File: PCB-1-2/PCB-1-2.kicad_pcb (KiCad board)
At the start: 2 copper layers, 51.3 x 8.4 mm, 37 parts, among them J1 Bus_PCI_Express_x8, U1 LTC1298IS8_PBF, U2 LTC1451IS8-PBF, U3 HI-3110PSIF, U4 FT231XS-R, U5 STM32F103RBT6, U6 STWD100YNXWY3F, U7 ADP7104ACPZ-5V, U8 ADP7104ACPZ-3.3V, Y1 8MHz Crystal

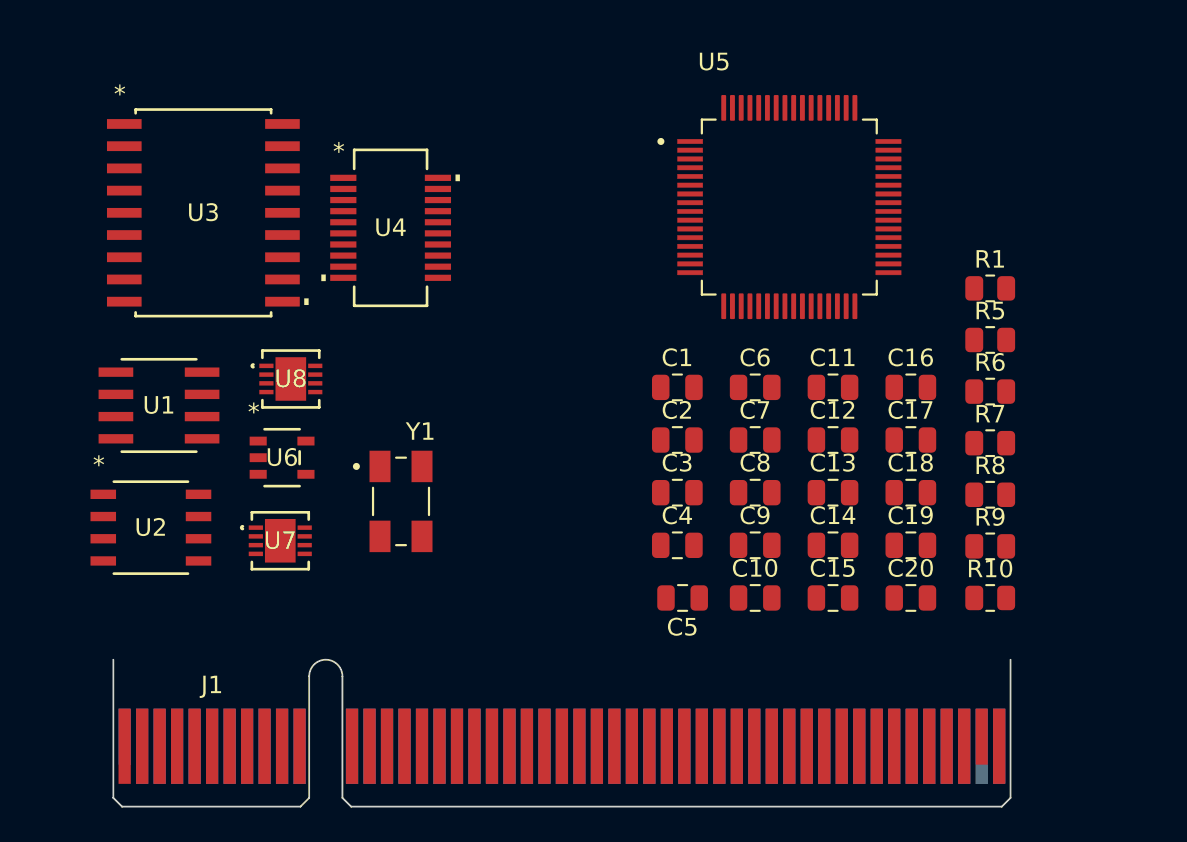
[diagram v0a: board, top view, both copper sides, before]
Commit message: Updated a few things
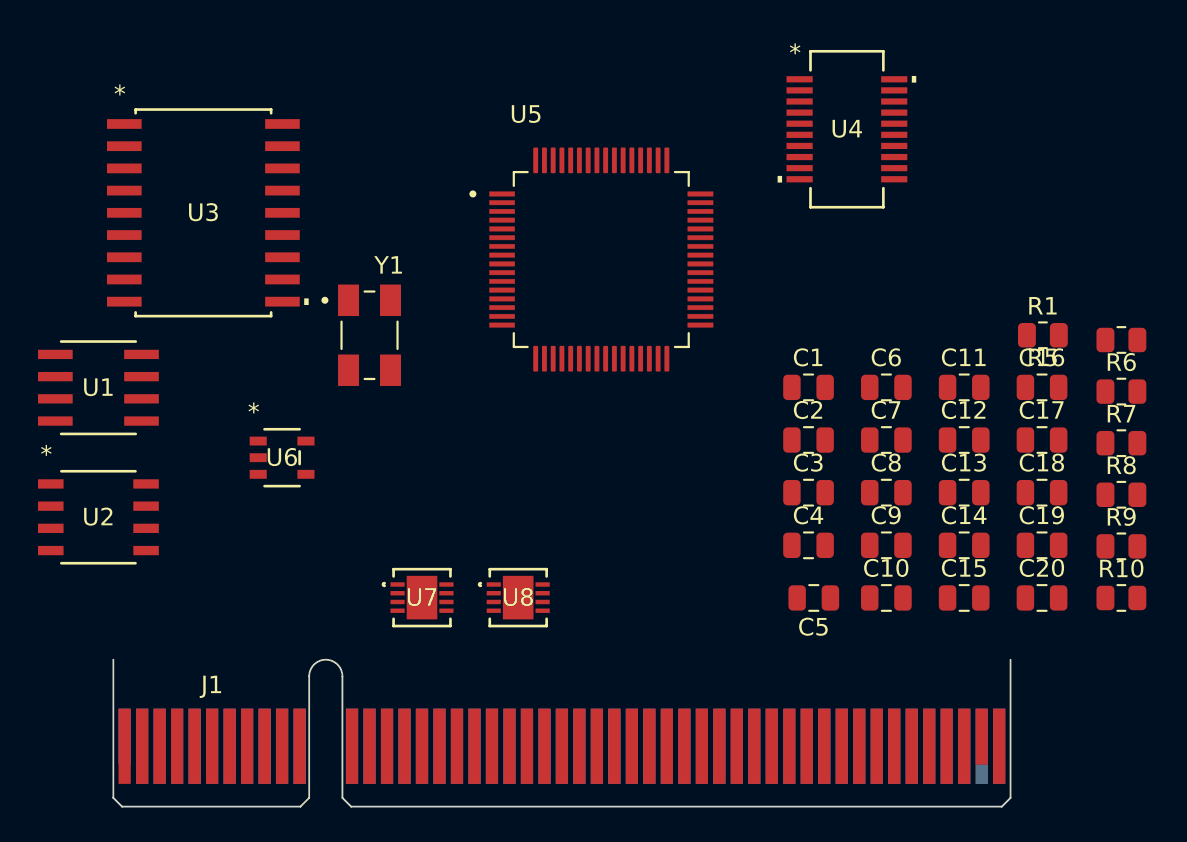
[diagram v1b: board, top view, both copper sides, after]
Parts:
- moved U4 26.7 mm to (71.3, 28.2)
- moved U8 18.0 mm to (52.5, 55.0)
- moved U5 11.2 mm to (57.2, 35.7)
- moved Y1 9.67 mm to (44.0, 40.0)
- moved U7 8.73 mm to (47.0, 55.0)
- moved C5 7.50 mm to (69.4, 55.0)
- moved C10 7.50 mm to (73.5, 55.0)
- moved C11 7.50 mm to (78.0, 43.0)
- moved C12 7.50 mm to (78.0, 46.0)
- moved C13 7.50 mm to (78.0, 49.0)
- moved C14 7.50 mm to (78.0, 52.0)
- moved C15 7.50 mm to (78.0, 55.0)
- moved C16 7.50 mm to (82.5, 43.0)
- moved C17 7.50 mm to (82.5, 46.0)
- moved C18 7.50 mm to (82.5, 49.0)
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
